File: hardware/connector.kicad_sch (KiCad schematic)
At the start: 2 parts, among them J1 Conn_02x10_Odd_Even, J2 Conn_01x05

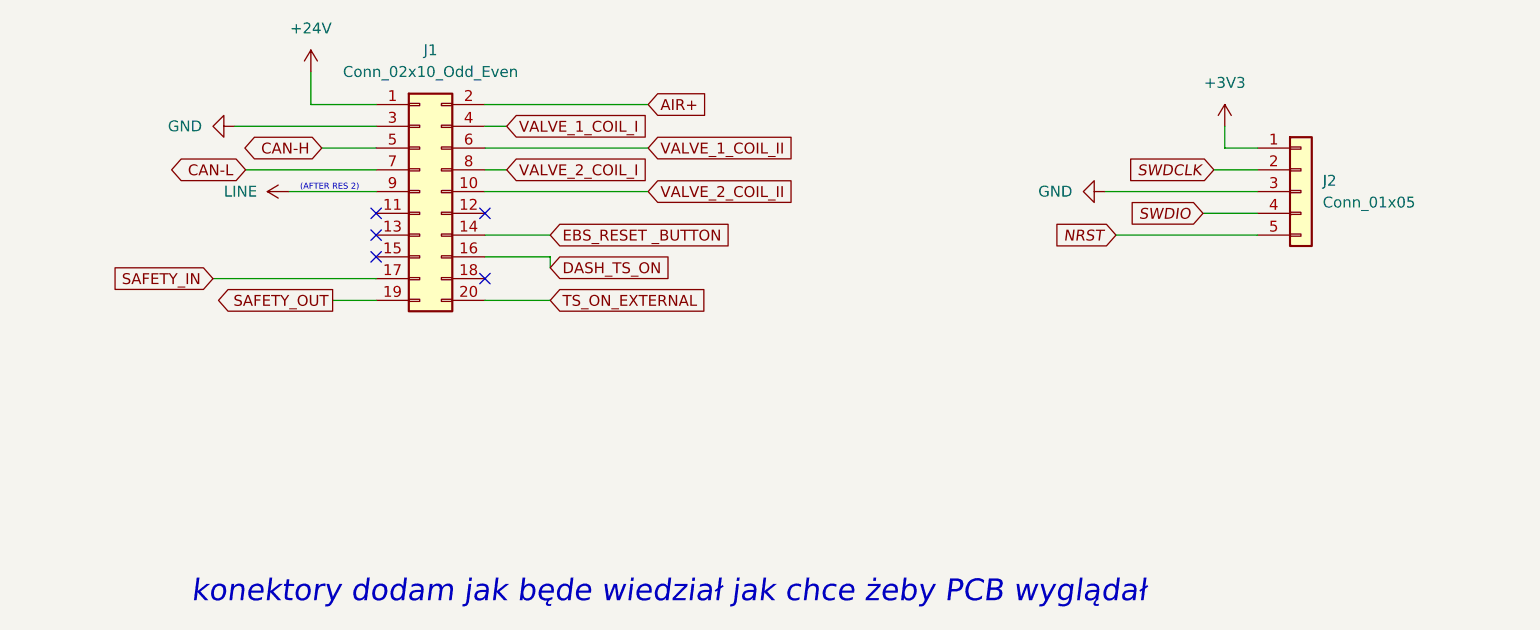
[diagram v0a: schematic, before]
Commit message: working simulations, assigned footprints
"nightly" relase
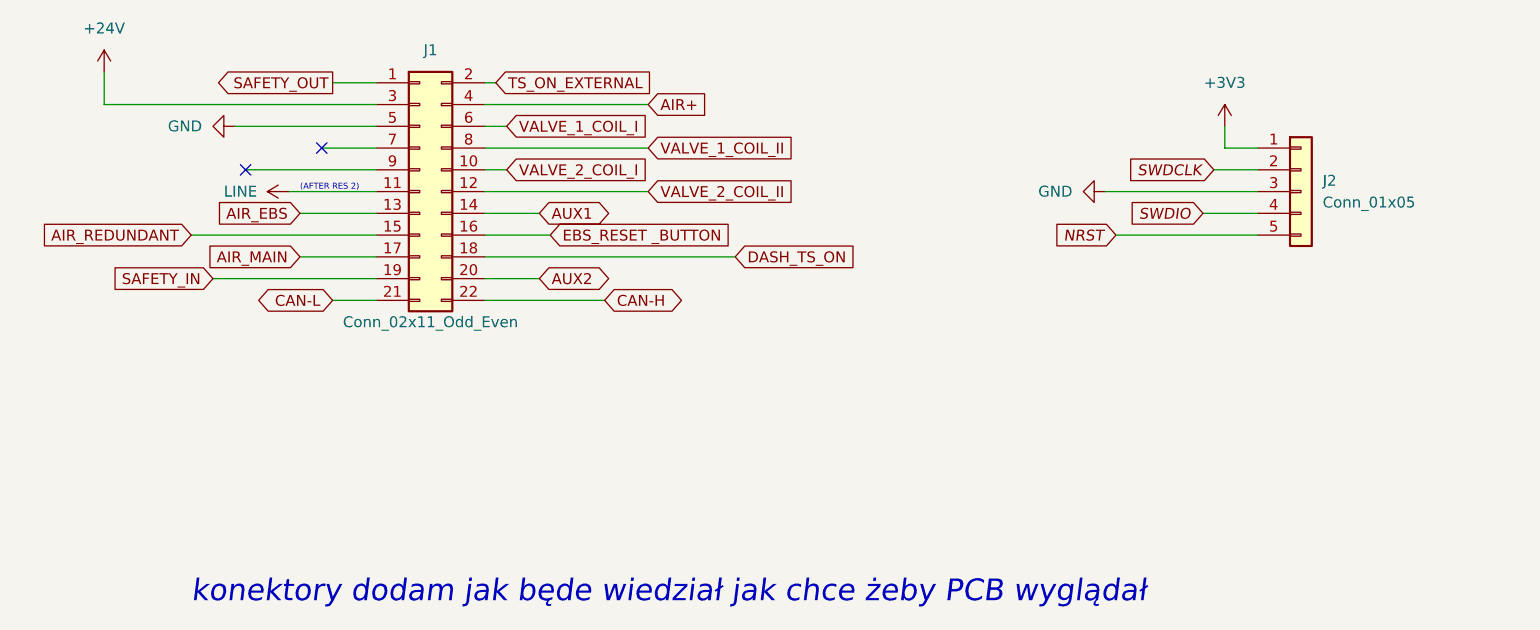
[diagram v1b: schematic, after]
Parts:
- J1: value Conn_02x10_Odd_Even -> Conn_02x11_Odd_Even; symbol Connector_Generic:Conn_02x10_Odd_Even -> Connector_Generic:Conn_02x11_Odd_Even
- J2: footprint (none) -> Connector_PinHeader_2.54mm:PinHeader_1x05_P2.54mm_Vertical
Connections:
- net +24V: now also J1.3 (Pin_3); no longer J1.1 (Pin_1)
- net AIR+: now also J1.4 (Pin_4); no longer J1.2 (Pin_2)
- net CAN-H: now also J1.22 (Pin_22); no longer J1.5 (Pin_5)
- net CAN-L: now also J1.21 (Pin_21); no longer J1.7 (Pin_7)
- net DASH_TS_ON: now also J1.18 (Pin_18); no longer J1.16 (Pin_16)
- net EBS_RESET _BUTTON: now also J1.16 (Pin_16); no longer J1.14 (Pin_14)
- net GND: now also J1.5 (Pin_5); no longer J1.3 (Pin_3)
- net LINE: now also J1.11 (Pin_11); no longer J1.9 (Pin_9)
- net SAFETY_IN: now also J1.19 (Pin_19); no longer J1.17 (Pin_17)
- net SAFETY_OUT: now also J1.1 (Pin_1); no longer J1.19 (Pin_19)
- net TS_ON_EXTERNAL: now also J1.2 (Pin_2); no longer J1.20 (Pin_20)
- net VALVE_1_COIL_I: now also J1.6 (Pin_6); no longer J1.4 (Pin_4)
- net VALVE_1_COIL_II: now also J1.8 (Pin_8); no longer J1.6 (Pin_6)
- net VALVE_2_COIL_I: now also J1.10 (Pin_10); no longer J1.8 (Pin_8)
- net VALVE_2_COIL_II: now also J1.12 (Pin_12); no longer J1.10 (Pin_10)
- net AIR_EBS: now reaches J1.13 (Pin_13)
- net AIR_REDUNDANT: now reaches J1.15 (Pin_15)
- new net AIR_MAIN: J1.17 (Pin_17)
- new net AUX1: J1.14 (Pin_14)
- new net AUX2: J1.20 (Pin_20)
- no-connect marks 5 -> 2
